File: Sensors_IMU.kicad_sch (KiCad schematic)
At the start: 19 parts, among them U19 ICM-20948, U20 KXTJ3-1057, U24 KX023-1025, U6 LSM303AH

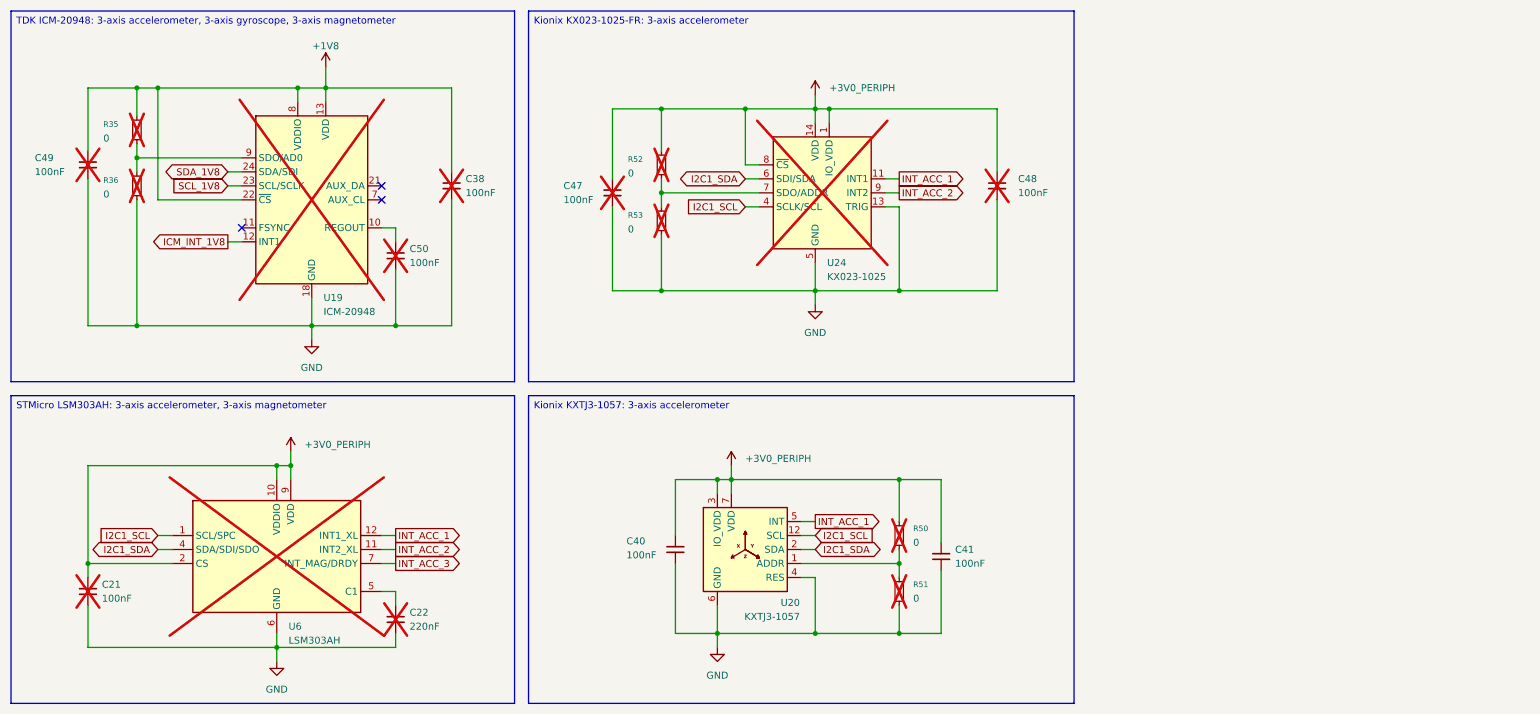
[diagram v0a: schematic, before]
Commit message: WIP: BOM
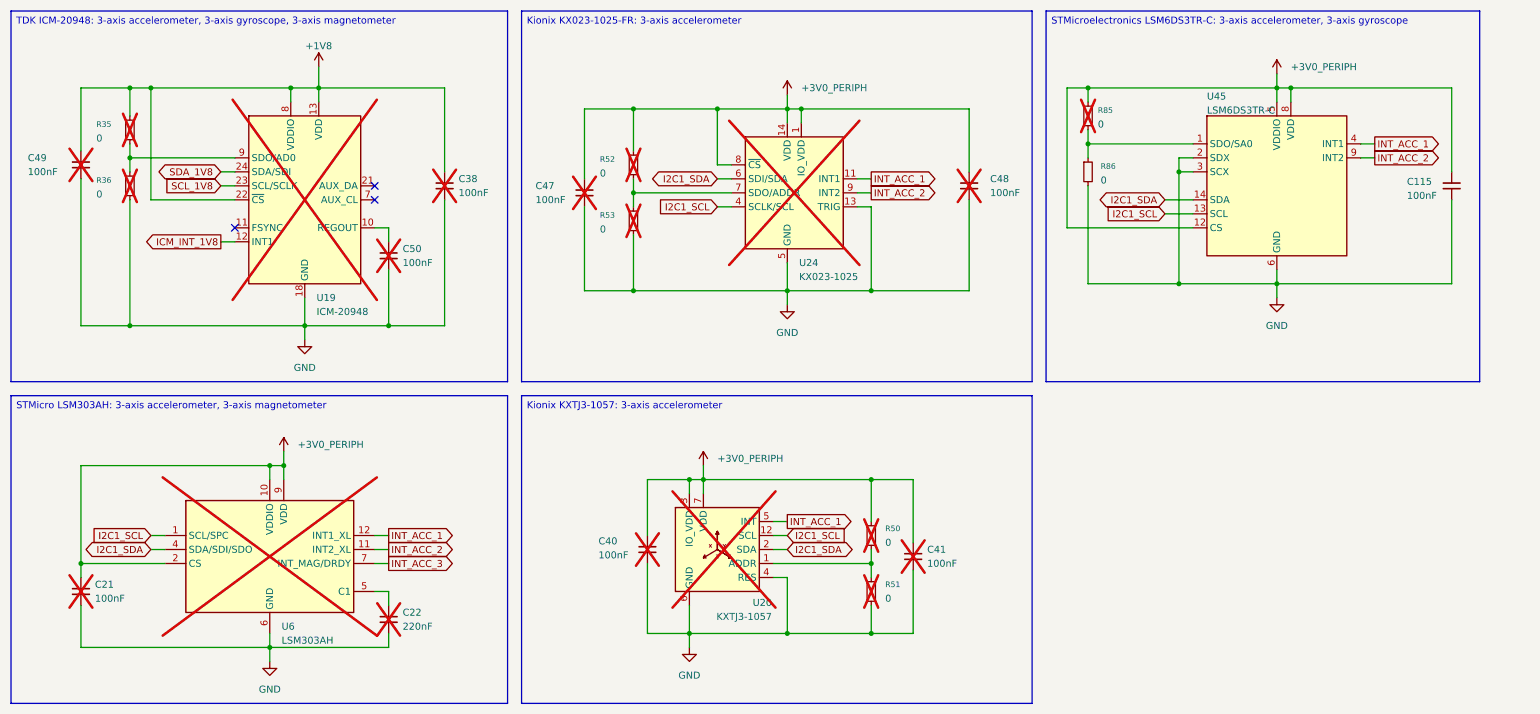
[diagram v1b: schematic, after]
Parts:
- added C115: 100nF, Capacitor_SMD:C_0402_1005Metric, symbol Device:C_Small
- added R85, R86: 0, Resistor_SMD:R_0402_1005Metric, symbol Device:R_Small
- added U45: LSM6DS3TR-C, Package_LGA:LGA-14_3x2.5mm_P0.5mm_LayoutBorder3x4y, symbol Sensor_Motion:LSM6DS3
- C21, C38, C47, C48, C49, C50: LCSC (none) -> C1525; now left out of the parts list
- C22: LCSC (none) -> C16772; now left out of the parts list
- C40, C41: LCSC (none) -> C1525; now not fitted; now left out of the parts list
- R35, R36, R52, R53: LCSC (none) -> C17168
- R50, R51: LCSC (none) -> C17168; now left out of the parts list
- U20: now not fitted; now left out of the parts list
- U24: LCSC (none) -> C236128
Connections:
- net +3V0_PERIPH: now also C115.1, R85.1, U45.12 (CS), U45.5 (VDDIO), U45.8 (VDD)
- net GND: now also C115.2, R86.2, U45.2 (SDX), U45.3 (SCX), U45.6 (GND), U45.7 (GND)
- net I2C1_SCL: now also U45.13 (SCL)
- net I2C1_SDA: now also U45.14 (SDA)
- net INT_ACC_1: now also U45.4 (INT1)
- net INT_ACC_2: now also U45.9 (INT2)
- new net: R85.2, R86.1, U45.1 (SDO/SA0)
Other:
- moved on the sheet: C21, C22, C38, C47, C48, C49, C50, R35, R36, R50, R51, R52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
